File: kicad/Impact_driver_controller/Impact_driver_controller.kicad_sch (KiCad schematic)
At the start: 35 parts, among them Q1 IRFP4468PbF, Q2 IRFP4468PbF, SW1 Reset, U1 Pico, U2 IR2104, U3 LM78M05, U4 LM78M12, U5 ACS712xLCTR-30A

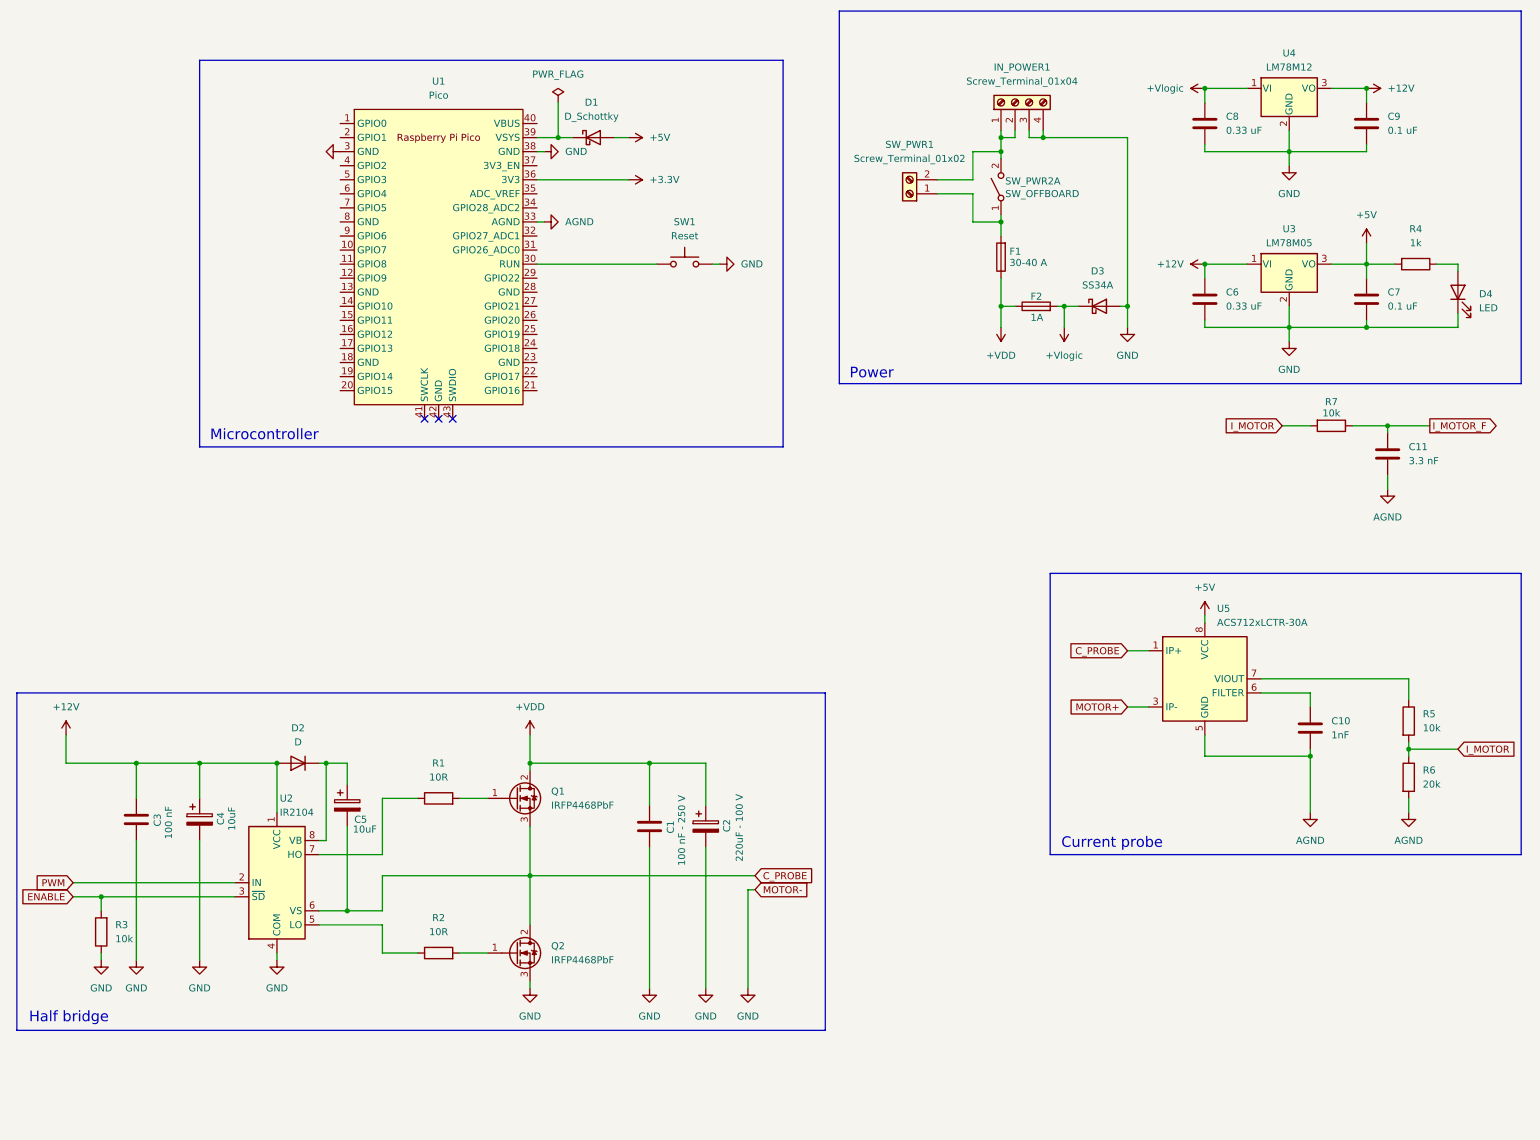
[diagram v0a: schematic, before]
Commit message: Add I/O
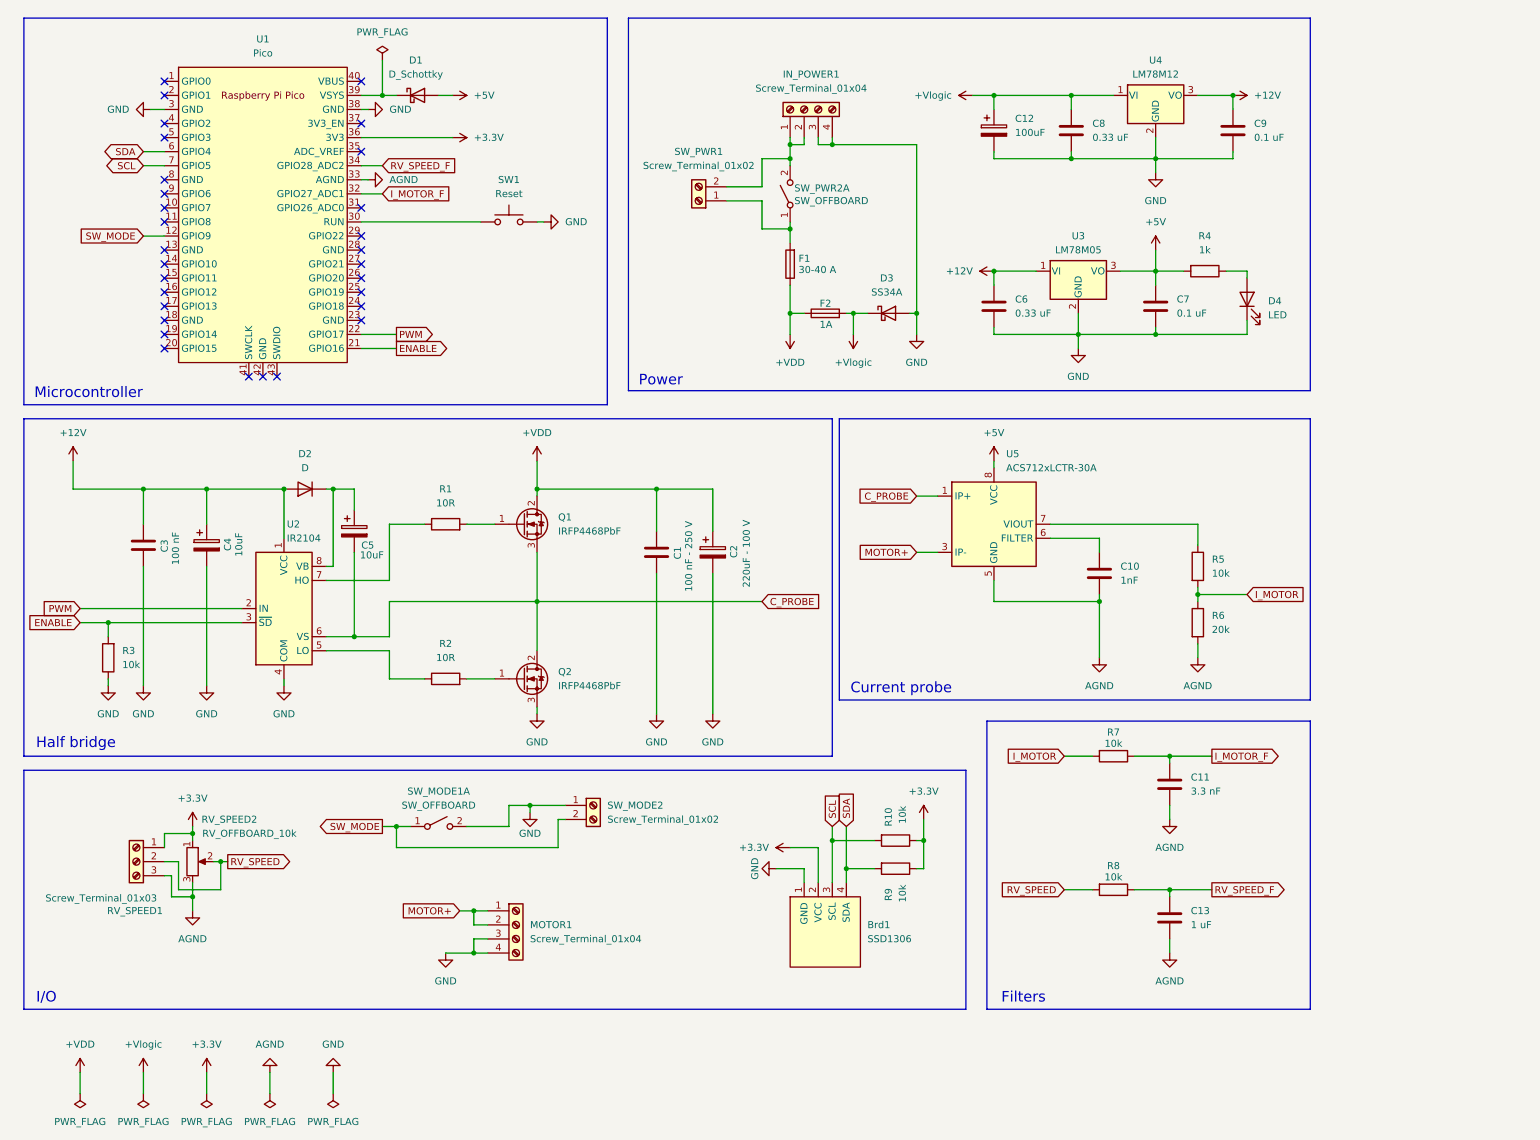
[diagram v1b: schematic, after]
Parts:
- added Brd1: SSD1306, SSD1306_impact:128x64OLED, symbol SSD1306-128x64_OLED_impact:SSD1306
- added C12: 100uF, Capacitor_SMD:CP_Elec_8x10, symbol Device:C_Polarized
- added C13: 1 uF, Capacitor_SMD:C_1206_3216Metric_Pad1.33x1.80mm_HandSolder, symbol Device:C
- added MOTOR1: Screw_Terminal_01x04, symbol Connector:Screw_Terminal_01x04
- added R10, R8, R9: 10k, Resistor_SMD:R_1206_3216Metric_Pad1.30x1.75mm_HandSolder, symbol Device:R
- added RV_SPEED1: Screw_Terminal_01x03, TerminalBlock_MetzConnect:TerminalBlock_MetzConnect_Type101_RT01603HBWC_1x03_P5.08mm_Horizontal, symbol Connector:Screw_Terminal_01x03
- added RV_SPEED2: RV_OFFBOARD_10k, symbol Device:R_Potentiometer
- added SW_MODE1: SW_OFFBOARD, symbol Switch:SW_DPST_x2
- added SW_MODE2: Screw_Terminal_01x02, TerminalBlock_MetzConnect:TerminalBlock_MetzConnect_Type101_RT01602HBWC_1x02_P5.08mm_Horizontal, symbol Connector:Screw_Terminal_01x02
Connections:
- net +3.3V: now also Brd1.2 (VCC), R10.1, R9.1, RV_SPEED1.1 (Pin_1), RV_SPEED2.1
- net +Vlogic: now also C12.1
- net AGND: now also C13.2, RV_SPEED1.3 (Pin_3), RV_SPEED2.3
- net ENABLE: now also U1.21 (GPIO16)
- net GND: now also Brd1.1 (GND), C12.2, MOTOR1.3 (Pin_3), MOTOR1.4 (Pin_4), SW_MODE1.2 (B), SW_MODE2.1 (Pin_1)
- net I_MOTOR_F: now also U1.32 (GPIO27_ADC1)
- net MOTOR+: now also MOTOR1.1 (Pin_1), MOTOR1.2 (Pin_2)
- net PWM: now also U1.22 (GPIO17)
- net SW_MODE: now reaches U1.12 (GPIO9)
- net SW_MODE: now also SW_MODE1.1 (A), SW_MODE2.2 (Pin_2)
- net RV_SPEED_F: now reaches U1.34 (GPIO28_ADC2)
- net RV_SPEED_F: now also C13.1, R8.1
- net SDA: now reaches U1.6 (GPIO4)
- net SDA: now also Brd1.4 (SDA), R9.2
- net SCL: now reaches U1.7 (GPIO5)
- net SCL: now also Brd1.3 (SCL), R10.2
- new net RV_SPEED: R8.2, RV_SPEED1.2 (Pin_2), RV_SPEED2.2
- no-connect marks 3 -> 30
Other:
- note added: "Filters"
- note added: "I/O"
- moved on the sheet: C1, C10, C11, C2, C3, C4, C5, C6, C7, C8, C9, D1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

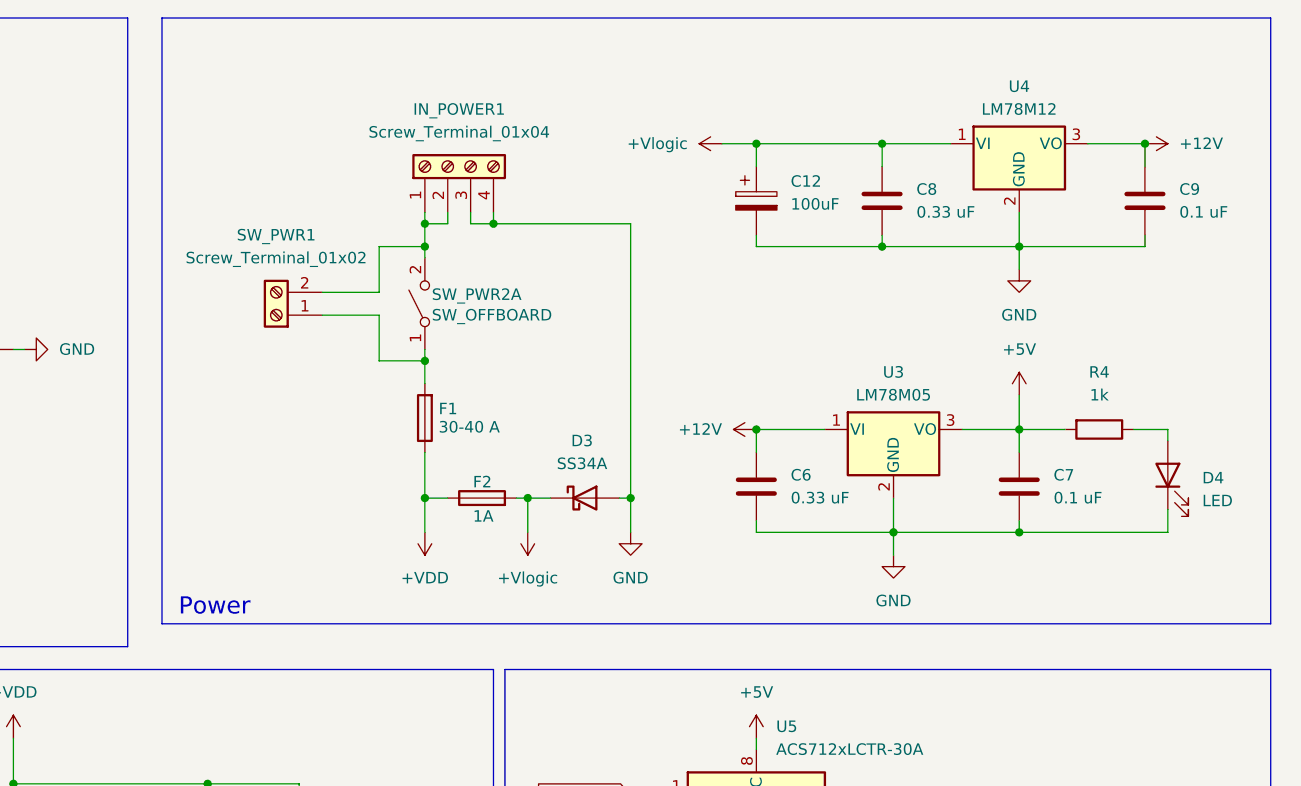
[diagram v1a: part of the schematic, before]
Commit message: Add MCU module
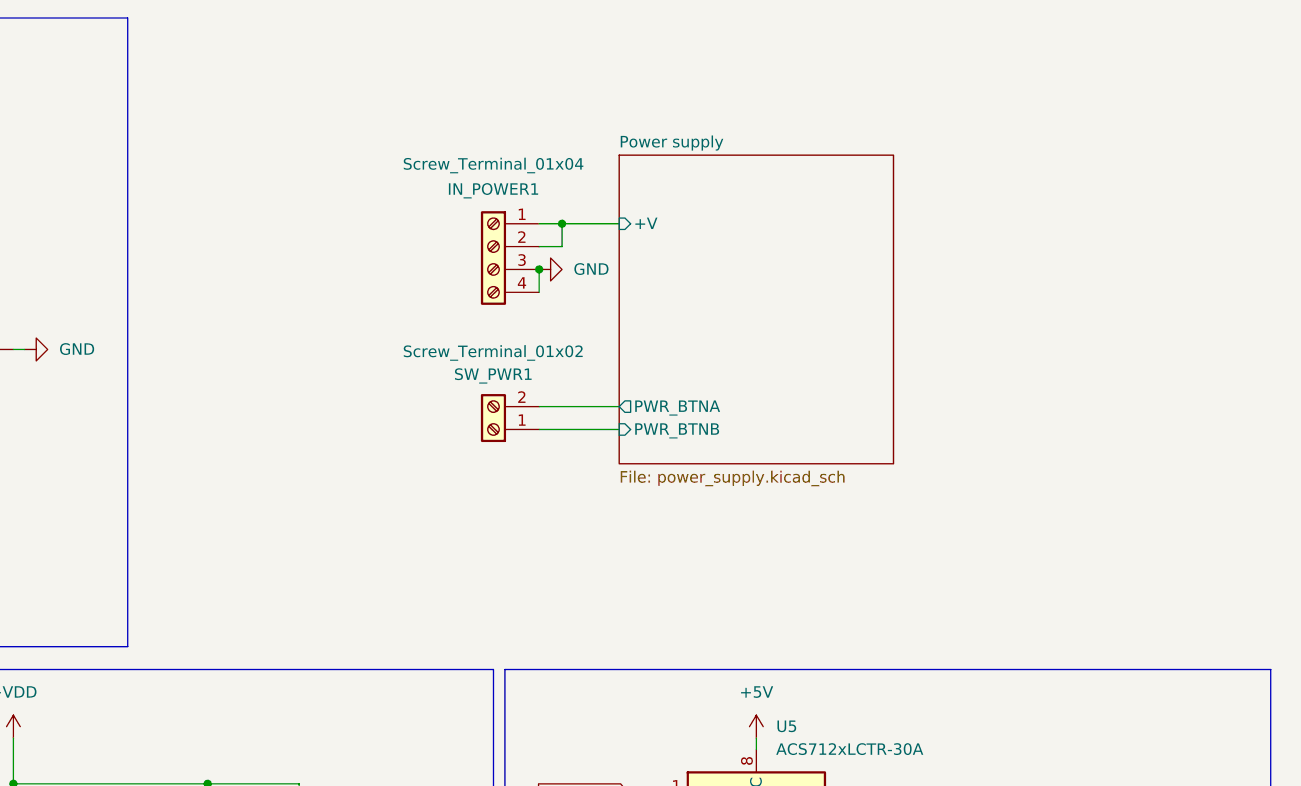
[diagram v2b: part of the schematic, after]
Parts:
- removed C12: 100uF, Capacitor_SMD:CP_Elec_8x10, symbol Device:C_Polarized
- removed C6, C8: 0.33 uF, Capacitor_SMD:C_1206_3216Metric_Pad1.33x1.80mm_HandSolder, symbol Device:C
- removed C7, C9: 0.1 uF, Capacitor_SMD:C_1206_3216Metric_Pad1.33x1.80mm_HandSolder, symbol Device:C
- removed D3: SS34A, Diode_SMD:D_SMB-SMC_Universal_Handsoldering, symbol Device:D_Schottky
- removed D4: LED, Diode_SMD:D_1206_3216Metric_Pad1.42x1.75mm_HandSolder, symbol Device:LED
- removed F1: 30-40 A, Fuse:Fuse_Blade_ATO_directSolder, symbol Device:Fuse
- removed F2: 1A, Fuse:Fuse_Blade_ATO_directSolder, symbol Device:Fuse
- removed R4: 1k, Resistor_SMD:R_1206_3216Metric_Pad1.30x1.75mm_HandSolder, symbol Device:R
- removed SW_PWR2: SW_OFFBOARD, symbol Switch:SW_DPST_x2
- removed U3: LM78M05, Package_TO_SOT_SMD:TO-252-2, symbol Regulator_Linear:LM78M05_TO252
- removed U4: LM78M12, Package_TO_SOT_SMD:TO-252-2, symbol Regulator_Linear:LM7812_TO220
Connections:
- net Power supply/+V: now reaches IN_POWER1.1 (Pin_1), IN_POWER1.2 (Pin_2)
- net Power supply/+V: no longer SW_PWR1.2 (Pin_2)
- net Power supply/PWR_BTNB: now reaches SW_PWR1.1 (Pin_1)
- new net Power supply/PWR_BTNA: SW_PWR1.2 (Pin_2)
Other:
- added sheet Power supply (power_supply.kicad_sch)
- note removed: "Power"
